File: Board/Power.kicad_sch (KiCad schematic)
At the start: 89 parts, among them J2 DCJ0202, Q4 IRLML5203

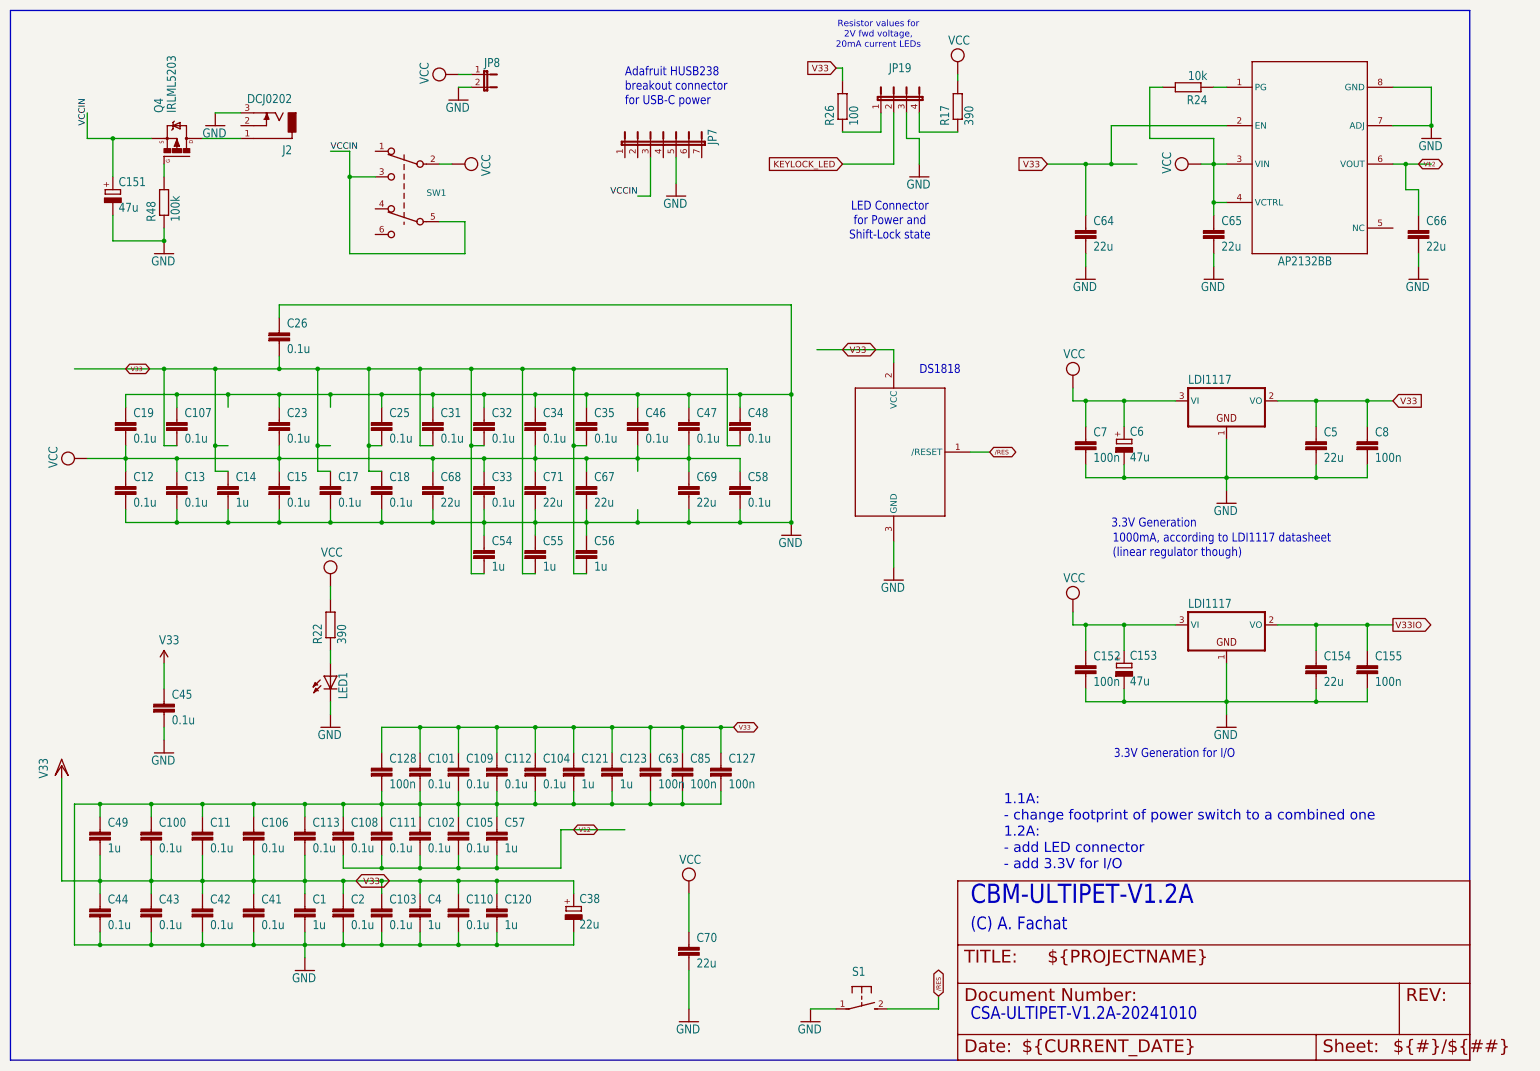
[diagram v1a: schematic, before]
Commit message: work on r1.3
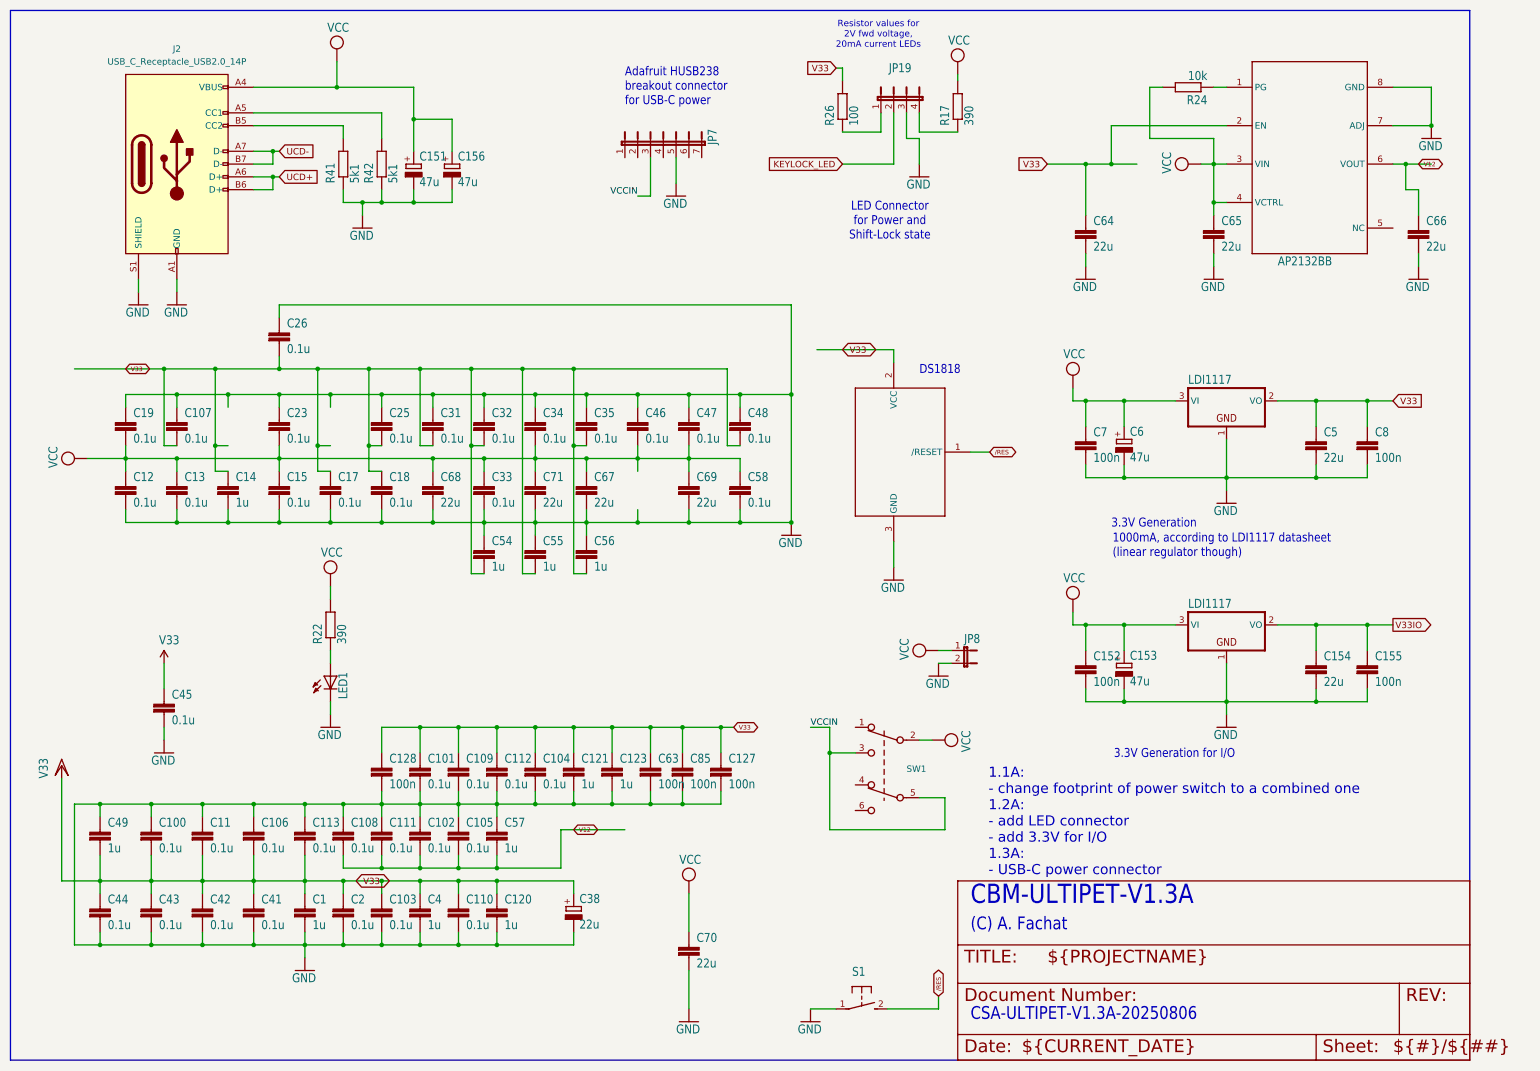
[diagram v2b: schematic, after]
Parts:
- removed C151: 47u, cbm_ultipet_v1:E2,5-6, symbol cbm_ultipet_v1-eagle-import:CPOL-EUE2.5-6
- removed J2: DCJ0202, cbm_ultipet_v1:DCJ0202, symbol cbm_ultipet_v1-eagle-import:DCJ0202
- removed Q4: IRLML5203, cbm_ultipet_v1:MICRO3, symbol cbm_ultipet_v1-eagle-import:IRLML5203
- removed R48: 100k, cbm_ultipet_v1:0207_2V, symbol cbm_ultipet_v1-eagle-import:R-EU_0207/2V
- added C151, C156: 47u, cbm_ultipet_v1:E2,5-6, symbol micropet_v3-eagle-import:CPOL-EUE5-6
- added J2: USB_C_Receptacle_USB2.0_14P, Connector_USB:USB_C_Receptacle_GCT_USB4085, symbol Connector:USB_C_Receptacle_USB2.0_14P
- added R41, R42: 5k1, cbm_ultipet_v1:0207_2V, symbol micropet_v3-eagle-import:R-EU_0207/2V
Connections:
- net GND: now also C151.-, C156.-, J2.A1 (GND), J2.A12 (GND), J2.B1 (GND), J2.B12 (GND), J2.S1 (SHIELD), R41.1, R42.1
- net VCC: now also C151.+, C156.+, J2.A4 (VBUS), J2.A9 (VBUS), J2.B4 (VBUS), J2.B9 (VBUS)
- new net: J2.A5 (CC1), R42.2
- new net: J2.B5 (CC2), R41.2
- new net UCD+: J2.A6 (D+), J2.B6 (D+)
- new net UCD-: J2.A7 (D-), J2.B7 (D-)
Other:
- note added: "1.1A: - change footprint of power switch to a combined one 1.2A: - add LED connector - add 3.3V for I/O 1.3A: - USB-C power connector"
- note added: "CBM-ULTIPET-V1.3A"
- note added: "CSA-ULTIPET-V1.3A-20250806"
- note removed: "1.1A: - change footprint of power switch to a combined one 1.2A: - add LED connector - add 3.3V for I/O"
- note removed: "CBM-ULTIPET-V1.2A"
- note removed: "CSA-ULTIPET-V1.2A-20241010"
- moved on the sheet: JP8, SW1

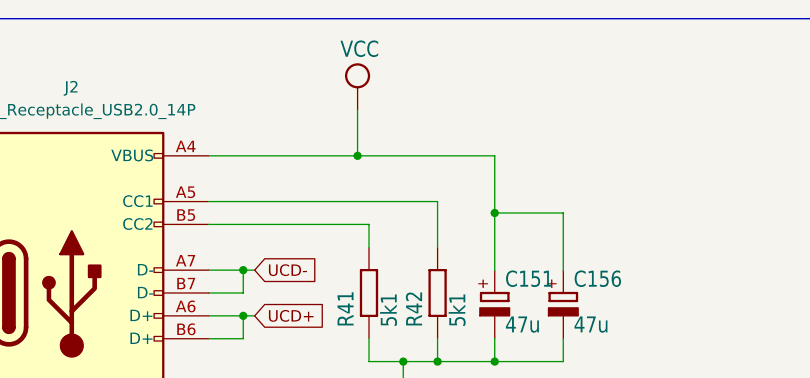
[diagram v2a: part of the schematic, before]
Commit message: more layout work on r1.3
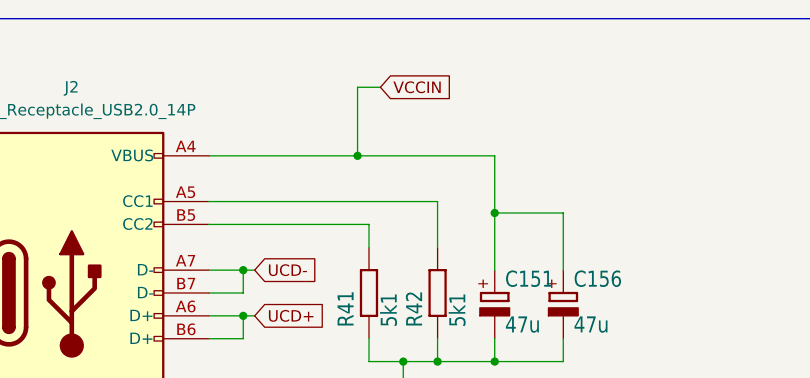
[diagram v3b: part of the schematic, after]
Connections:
- net VCC: no longer C151.+, C156.+, J2.A4 (VBUS), J2.A9 (VBUS), J2.B4 (VBUS), J2.B9 (VBUS)
- net VCCIN: now also C151.+, C156.+, J2.A4 (VBUS), J2.A9 (VBUS), J2.B4 (VBUS), J2.B9 (VBUS)
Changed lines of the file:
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@@
 	(wire
 		(pts
+			(xy 82.55 25.4) (xy 82.55 33.02)
+		)
+		(stroke
+			(width 0)
+			(type default)
+		)
+	)
+	(wire
+		(pts
 			(xy 132.08 96.52) (xy 132.08 93.98)
 		)
@@
 	(wire
 		(pts
+			(xy 85.09 25.4) (xy 82.55 25.4)
+		)
+		(stroke
+			(width 0)
+			(type default)
+		)
+	)
+	(wire
+		(pts
 			(xy 97.79 45.72) (xy 97.79 39.37)
 		)
@@
 	(wire
 		(pts
-			(xy 82.55 27.94) (xy 82.55 33.02)
-		)
-		(stroke
-			(width 0)
-			(type default)
-		)
-	)
-	(wire
-		(pts
 			(xy 106.68 187.96) (xy 114.3 187.96)
 		)
@@
 		)
 	)
+	(global_label "VCCIN"
+		(shape input)
+		(at 85.09 25.4 0)
+		(fields_autoplaced yes)
+		(effects
+			(font
+				(size 1.27 1.27)
+			)
+			(justify left)
+		)
+		(property "Intersheetrefs" "${INTERSHEET_REFS}"
+			(at 93.6391 25.4 0)
+			(effects
+				(font
+					(size 1.27 1.27)
+				)
+				(justify left)
+				(hide yes)
+			)
+		)
+	)
 	(global_label "V12"
 		(shape bidirectional)
@@
 					(unit 1)
 				)
-			)
-		)
-	)
-	(symbol
-		(lib_id "micropet_v3-eagle-import:VCC")
-		(at 82.55 25.4 0)
-		(unit 1)
-		(exclude_from_sim no)
-		(in_bom yes)
-		(on_board yes)
-		(dnp no)
-		(property "Reference" "#V049"
-			(at 82.55 25.4 0)
-			(effects
-				(font
-					(size 1.27 1.27)
-				)
-				(hide yes)
-			)
-		)
-		(property "Value" "VCC"
-			(at 80.645 22.225 0)
-			(effects
-				(font
-					(size 1.778 1.5113)
-				)
-				(justify left bottom)
-			)
-		)
-		(property "Footprint" ""
-			(at 82.55 25.4 0)
-			(effects
-				(font
-					(size 1.27 1.27)
-				)
-				(hide yes)
-			)
-		)
-		(property "Datasheet" ""
-			(at 82.55 25.4 0)
-			(effects
-				(font
-					(size 1.27 1.27)
-				)
-				(hide yes)
-			)
-		)
-		(property "Description" ""
-			(at 82.55 25.4 0)
-			(effects
-				(font
-					(size 1.27 1.27)
-				)
-				(hide yes)
-			)
-		)
-		(pin "1"
-		)
-		(instances
-			(project "cbm_ultipet_v1"
-				(path "/4dd2dd78-173f-4b46-8cce-4ed940435c94/f2a7836e-baa5-4eed-9e59-e26d91b4d1a6"
-					(reference "#V049")
-					(unit 1)
-				)
